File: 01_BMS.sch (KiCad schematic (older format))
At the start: 51 parts, among them J201 TB001-500-07BE CUI_Devices, Q201 NTD14N03RT4G, Q202 NTD14N03RT4G, Q203 NTD14N03RT4G, U201 BQ76920, U202 BQ76200

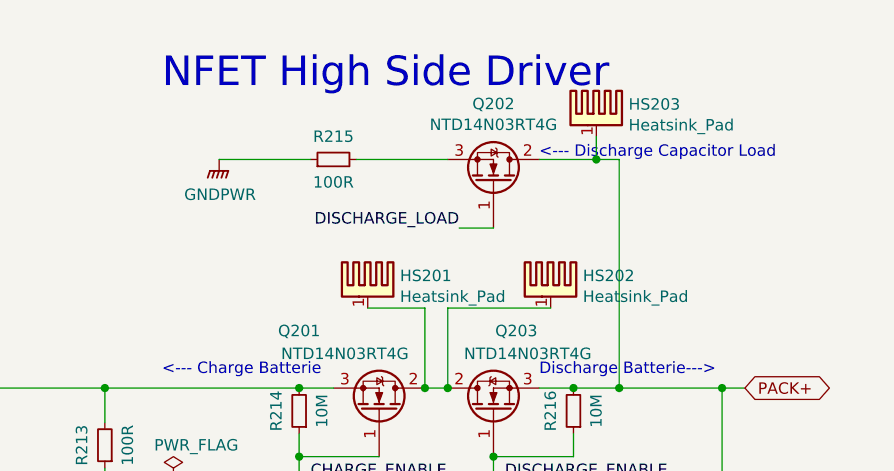
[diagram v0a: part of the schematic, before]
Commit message: fertig zum routen
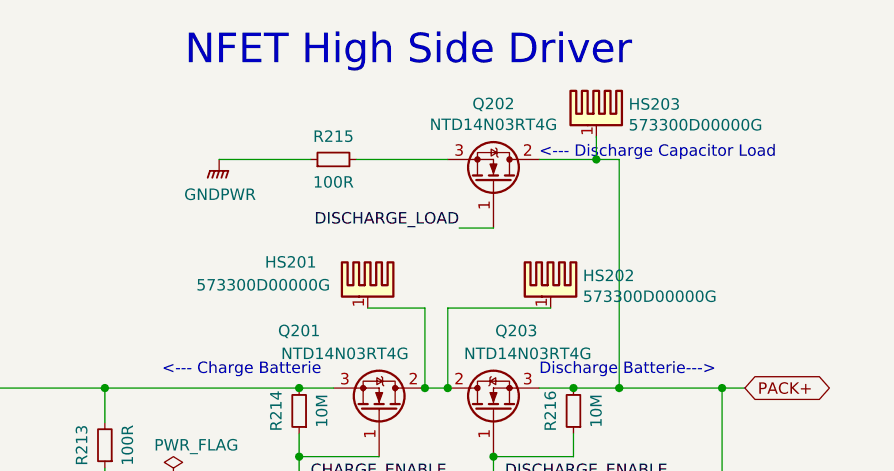
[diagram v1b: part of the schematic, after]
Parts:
- HS201, HS202, HS203: value Heatsink_Pad -> 573300D00000G
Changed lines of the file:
@@
 Text Notes 4650 1550 0    129  ~ 0
 Battery Balancer
-Text Notes 8200 850  0    129  ~ 0
+Text Notes 8300 750  0    129  ~ 0
 NFET High Side Driver
 Text GLabel 10050 3700 2    50   Input ~ 0
@@
 AR Path="/5E73BADE/5E9AC02A" Ref="HS203"  Part="1"
 F 0 "HS203" H 10241 991 50  0000 L CNN
-F 1 "Heatsink_Pad" H 10241 900 50  0000 L CNN
+F 1 "573300D00000G" H 10241 900 50  0000 L CNN
 F 2 "Heatsink:Heatsink_AAVID_573300D00010G_TO-263" H 10112 900 50  0001 C CNN
-F 3 "~" H 10112 900 50  0001 C CNN
+F 3 "https://www.mouser.de/datasheet/2/2/Aavid-Board-Level-Heatsinks-Catalog-2018-1507171.pdf" H 10112 900 50  0001 C CNN
 	1    10100 950
 	1    0    0    -1
@@
 AR Path="/5E73BAE8/5E9B8E57" Ref="HS?"  Part="1"
 AR Path="/5E73BADE/5E9B8E57" Ref="HS201"  Part="1"
-F 0 "HS201" H 9241 1741 50  0000 L CNN
-F 1 "Heatsink_Pad" H 9241 1650 50  0000 L CNN
+F 0 "HS201" H 8650 1800 50  0000 L CNN
+F 1 "573300D00000G" H 8350 1700 50  0000 L CNN
 F 2 "Heatsink:Heatsink_AAVID_573300D00010G_TO-263" H 9112 1650 50  0001 C CNN
-F 3 "~" H 9112 1650 50  0001 C CNN
+F 3 "https://www.mouser.de/datasheet/2/2/Aavid-Board-Level-Heatsinks-Catalog-2018-1507171.pdf" H 9112 1650 50  0001 C CNN
 	1    9100 1700
 	1    0    0    -1
@@
 AR Path="/5E73BADE/5E9BEE65" Ref="HS202"  Part="1"
 F 0 "HS202" H 10041 1741 50  0000 L CNN
-F 1 "Heatsink_Pad" H 10041 1650 50  0000 L CNN
+F 1 "573300D00000G" H 10041 1650 50  0000 L CNN
 F 2 "Heatsink:Heatsink_AAVID_573300D00010G_TO-263" H 9912 1650 50  0001 C CNN
-F 3 "~" H 9912 1650 50  0001 C CNN
+F 3 "https://www.mouser.de/datasheet/2/2/Aavid-Board-Level-Heatsinks-Catalog-2018-1507171.pdf" H 9912 1650 50  0001 C CNN
 	1    9900 1700
 	1    0    0    -1
